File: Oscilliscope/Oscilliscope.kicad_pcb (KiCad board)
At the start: 2 copper layers, 56 x 32 mm, 48 parts, among them J1 SPI1, J10 TFT_PWR, J2 USART, J3 USB_B_Micro, J4 SPI1, J5 Conn_01x02_Pin, J6 SWD, J7 Conn_01x02_Pin, J8 Conn_01x02_Pin, J9 SIG_IN, U1 AMS1117-3.3, U2 STM32F411CEU6, U3 MCP6022, Y1 25mHz

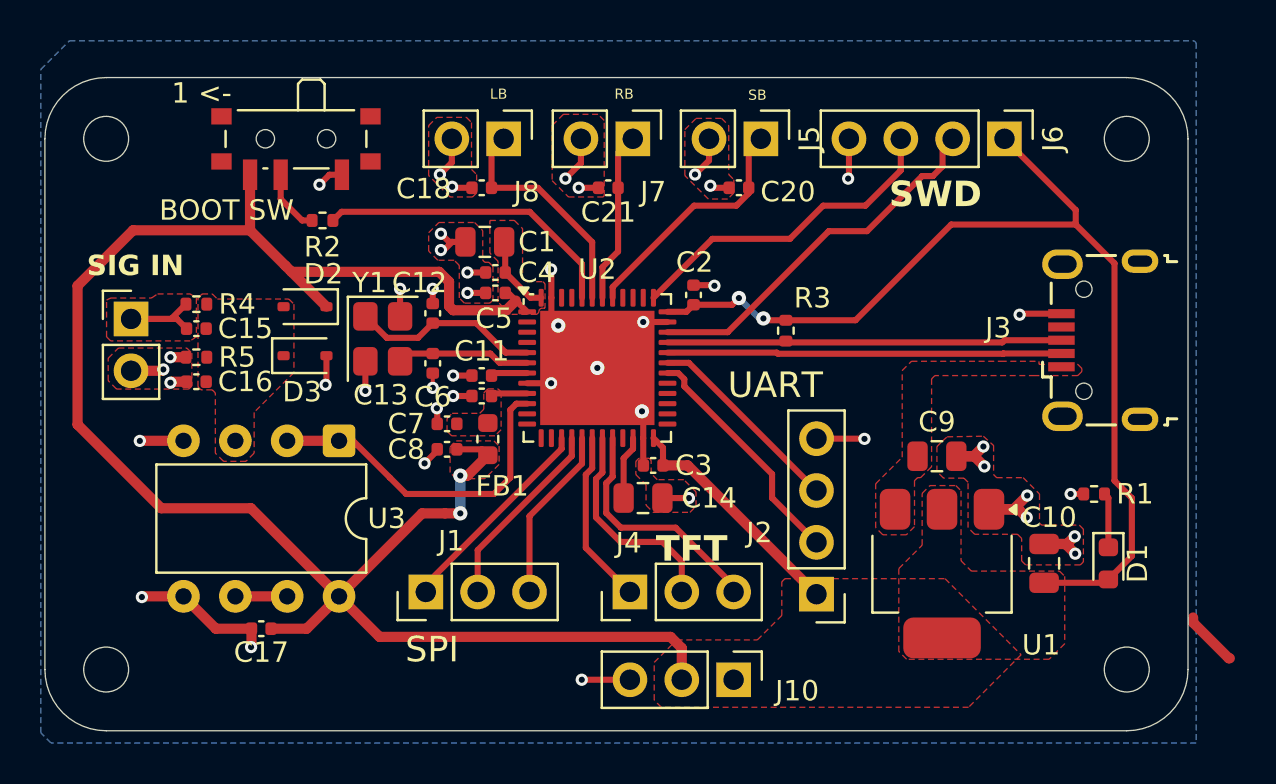
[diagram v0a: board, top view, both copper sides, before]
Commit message: PCB Update
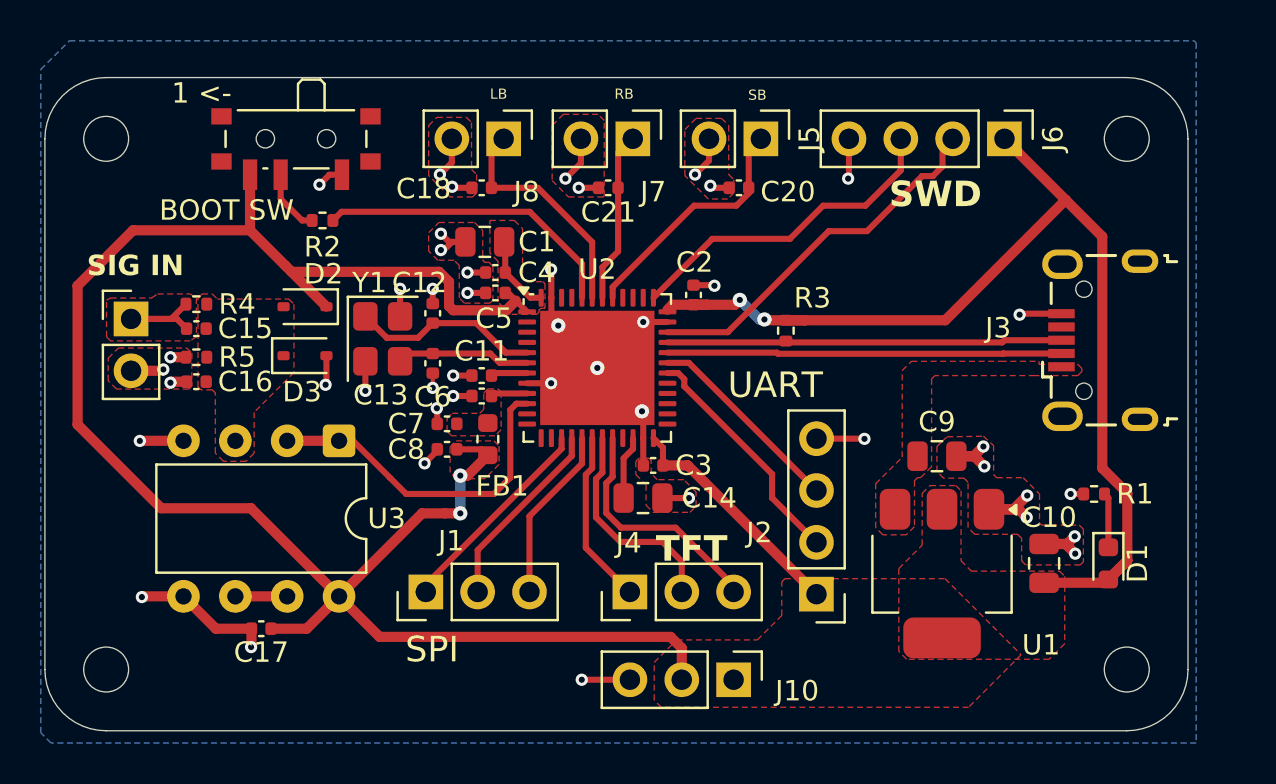
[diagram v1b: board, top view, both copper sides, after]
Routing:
- net +3.3V: track 157.7 -> 160.5 mm
- net (no net): track 2.77 -> 0.00 mm
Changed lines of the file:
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@@
-	)
-	(segment
-		(start 153.25 115.65)
-		(end 153.2 115.65)
-		(width 0.5)
-		(layer "F.Cu")
-		(net 0)
-	)
-	(segment
-		(start 151.451 113.901)
-		(end 151.451 113.65)
-		(width 0.5)
-		(layer "F.Cu")
-		(net 0)
-	)
-	(segment
-		(start 153.2 115.65)
-		(end 151.451 113.901)
-		(width 0.5)
-		(layer "F.Cu")
-		(net 0)
 	)
 	(segment
@@
 	)
 	(segment
-		(start 128.87 98.33)
-		(end 126.975 98.33)
-		(width 0.3)
-		(layer "F.Cu")
-		(net 2)
-	)
-	(segment
 		(start 133 112.51)
 		(end 126.69 106.2)
@@
 	)
 	(segment
+		(start 148.226 110.8615)
+		(end 147.3 111.7875)
+		(width 0.5)
+		(layer "F.Cu")
+		(net 2)
+	)
+	(segment
 		(start 126.4 115.15)
 		(end 125.85 114.6)
@@
 	)
 	(segment
-		(start 145.699 93.689)
-		(end 142.21 90.2)
-		(width 0.3)
-		(layer "F.Cu")
-		(net 2)
-	)
-	(segment
 		(start 115 97.2)
 		(end 115 98.4)
@@
 	)
 	(segment
+		(start 142.21 90.2)
+		(end 145.205 93.195)
+		(width 0.5)
+		(layer "F.Cu")
+		(net 2)
+	)
+	(segment
 		(start 118.9875 97.9875)
 		(end 117.75 96.75)
@@
 	)
 	(segment
+		(start 145.205 93.195)
+		(end 139.31 99.09)
+		(width 0.5)
+		(layer "F.Cu")
+		(net 2)
+	)
+	(segment
+		(start 147.001 106.338528)
+		(end 148.226 107.563528)
+		(width 0.5)
+		(layer "F.Cu")
+		(net 2)
+	)
+	(segment
+		(start 127.65 98.33)
+		(end 125.944 98.33)
+		(width 0.5)
+		(layer "F.Cu")
+		(net 2)
+	)
+	(segment
 		(start 116.6125 105.4125)
 		(end 116.9 105.7)
@@
 	)
 	(segment
-		(start 145.699 94.4)
-		(end 139.6 94.4)
-		(width 0.3)
+		(start 147.001 94.991)
+		(end 147.001 106.338528)
+		(width 0.5)
+		(layer "F.Cu")
+		(net 2)
+	)
+	(segment
+		(start 129.242525 98.092525)
+		(end 129.00505 98.33)
+		(width 0.5)
 		(layer "F.Cu")
 		(net 2)
@@
 	)
 	(segment
+		(start 132.45 99.09)
+		(end 131.5 99.09)
+		(width 0.5)
+		(layer "F.Cu")
+		(net 2)
+	)
+	(segment
 		(start 109.61 112.615)
 		(end 113.675 108.55)
@@
 	)
 	(segment
-		(start 148.45 107.8)
-		(end 147.599 106.949)
-		(width 0.3)
-		(layer "F.Cu")
-		(net 2)
-	)
-	(segment
 		(start 113.675 108.55)
 		(end 114.8 108.55)
@@
 	)
 	(segment
-		(start 144.15 111.95)
-		(end 147.1375 111.95)
-		(width 0.3)
-		(layer "F.Cu")
-		(net 2)
-	)
-	(segment
 		(start 99.5175 94.6825)
 		(end 105.25 94.6825)
@@
 	)
 	(segment
+		(start 130.49 99.09)
+		(end 130.45 99.05)
+		(width 0.5)
+		(layer "F.Cu")
+		(net 2)
+	)
+	(segment
 		(start 114.51625 96.71625)
 		(end 115 97.2)
@@
 	)
 	(segment
-		(start 126.63 98.675)
-		(end 126.975 98.33)
-		(width 0.3)
+		(start 129.00505 98.33)
+		(end 127.65 98.33)
+		(width 0.5)
+		(layer "F.Cu")
+		(net 2)
+	)
+	(segment
+		(start 148.226 110.8615)
+		(end 147.1375 111.95)
+		(width 0.5)
+		(layer "F.Cu")
+		(net 2)
+	)
+	(segment
+		(start 147.1375 111.95)
+		(end 144.15 111.95)
+		(width 0.5)
 		(layer "F.Cu")
 		(net 2)
@@
 	)
 	(segment
-		(start 147.599 96.3)
-		(end 145.699 94.4)
-		(width 0.3)
+		(start 125.944 98.33)
+		(end 125.7 98.574)
+		(width 0.5)
 		(layer "F.Cu")
 		(net 2)
@@
 	)
 	(segment
-		(start 131.5 99.09)
-		(end 130.49 99.09)
-		(width 0.3)
-		(layer "F.Cu")
-		(net 2)
-	)
-	(segment
-		(start 125.7 98.675)
-		(end 126.63 98.675)
-		(width 0.3)
-		(layer "F.Cu")
-		(net 2)
-	)
-	(segment
 		(start 117.75 96.75)
 		(end 117.75 95.3)
@@
 	)
 	(segment
+		(start 148.226 107.563528)
+		(end 148.226 110.8615)
+		(width 0.5)
+		(layer "F.Cu")
+		(net 2)
+	)
+	(segment
 		(start 115.55 106.7)
 		(end 115.9 106.7)
@@
 	)
 	(segment
-		(start 148.45 110.6375)
-		(end 148.45 107.8)
-		(width 0.3)
-		(layer "F.Cu")
-		(net 2)
-	)
-	(segment
-		(start 129.2 98)
-		(end 128.87 98.33)
-		(width 0.3)
-		(layer "F.Cu")
-		(net 2)
-	)
-	(segment
-		(start 147.3 111.7875)
-		(end 148.45 110.6375)
-		(width 0.3)
+		(start 139.31 99.09)
+		(end 132.45 99.09)
+		(width 0.5)
+		(layer "F.Cu")
+		(net 2)
+	)
+	(segment
+		(start 132.45 99.09)
+		(end 130.49 99.09)
+		(width 0.5)
 		(layer "F.Cu")
 		(net 2)
@@
 	)
 	(segment
-		(start 147.599 106.949)
-		(end 147.599 96.3)
-		(width 0.3)
+		(start 145.205 93.195)
+		(end 147.001 94.991)
+		(width 0.5)
 		(layer "F.Cu")
 		(net 2)
@@
 	)
 	(segment
-		(start 130.49 99.09)
-		(end 130.4 99)
-		(width 0.3)
-		(layer "F.Cu")
-		(net 2)
-	)
-	(segment
 		(start 106.98375 96.41625)
 		(end 105.25 94.6825)
@@
 	)
 	(segment
+		(start 127.65 98.33)
+		(end 126.975 98.33)
+		(width 0.5)
+		(layer "F.Cu")
+		(net 2)
+	)
+	(segment
 		(start 107.28375 96.71625)
 		(end 114.51625 96.71625)
@@
 	)
 	(segment
-		(start 145.699 94.4)
-		(end 145.699 93.689)
-		(width 0.3)
-		(layer "F.Cu")
-		(net 2)
-	)
-	(segment
 		(start 114.8 108.55)
 		(end 115.55 108.55)
@@
 	)
 	(segment
-		(start 134.91 99.09)
-		(end 131.5 99.09)
-		(width 0.3)
-		(layer "F.Cu")
-		(net 2)
-	)
-	(segment
 		(start 108.025 114.2)
 		(end 109.61 112.615)
@@
 	)
 	(segment
-		(start 139.6 94.4)
-		(end 134.91 99.09)
-		(width 0.3)
-		(layer "F.Cu")
-		(net 2)
-	)
-	(segment
 		(start 96.8 104.2)
 		(end 96.8 97.4)
@@
 	)
 	(via
-		(at 130.4 99)
+		(at 129.242525 98.092525)
+		(size 0.7)
+		(drill 0.3)
+		(layers "F.Cu" "B.Cu")
+		(net 2)
+	)
+	(via
+		(at 130.45 99.05)
 		(size 0.7)
 		(drill 0.3)
@@
 		(net 2)
 	)
-	(via
-		(at 129.2 98)
-		(size 0.7)
-		(drill 0.3)
-		(layers "F.Cu" "B.Cu")
-		(net 2)
-	)
-	(segment
-		(start 130.2 99)
-		(end 129.2 98)
-		(width 0.3)
-		(layer "B.Cu")
-		(net 2)
-	)
 	(segment
 		(start 115.55 108.55)
@@
 	)
 	(segment
-		(start 130.4 99)
-		(end 130.2 99)
-		(width 0.3)
+		(start 130.45 99.05)
+		(end 130.2 99.05)
+		(width 0.5)
+		(layer "B.Cu")
+		(net 2)
+	)
+	(segment
+		(start 130.2 99.05)
+		(end 129.242525 98.092525)
+		(width 0.5)
 		(layer "B.Cu")
 		(net 2)
@@
 		(polygon
 			(pts
-				(xy 139.3 111.75) (xy 143.025 115.475) (xy 143.025 115.475) (xy 140.45 118.05) (xy 125.4 118.05)
-				(xy 125.05 117.7) (xy 125.05 115.85) (xy 126.15 114.75) (xy 130.1 114.75) (xy 131.3 113.55) (xy 131.3 111.9)
-				(xy 131.45 111.75)
+				(xy 139.3 111.75) (xy 143.025 115.475) (xy 140.45 118.05) (xy 125.4 118.05) (xy 125.05 117.7) (xy 125.05 115.85)
+				(xy 126.15 114.75) (xy 130.1 114.75) (xy 131.3 113.55) (xy 131.3 111.9) (xy 131.45 111.75)
 			)
 		)
